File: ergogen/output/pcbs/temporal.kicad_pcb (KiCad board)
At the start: 2 copper layers, 147.9 x 107.9 mm, 57 parts

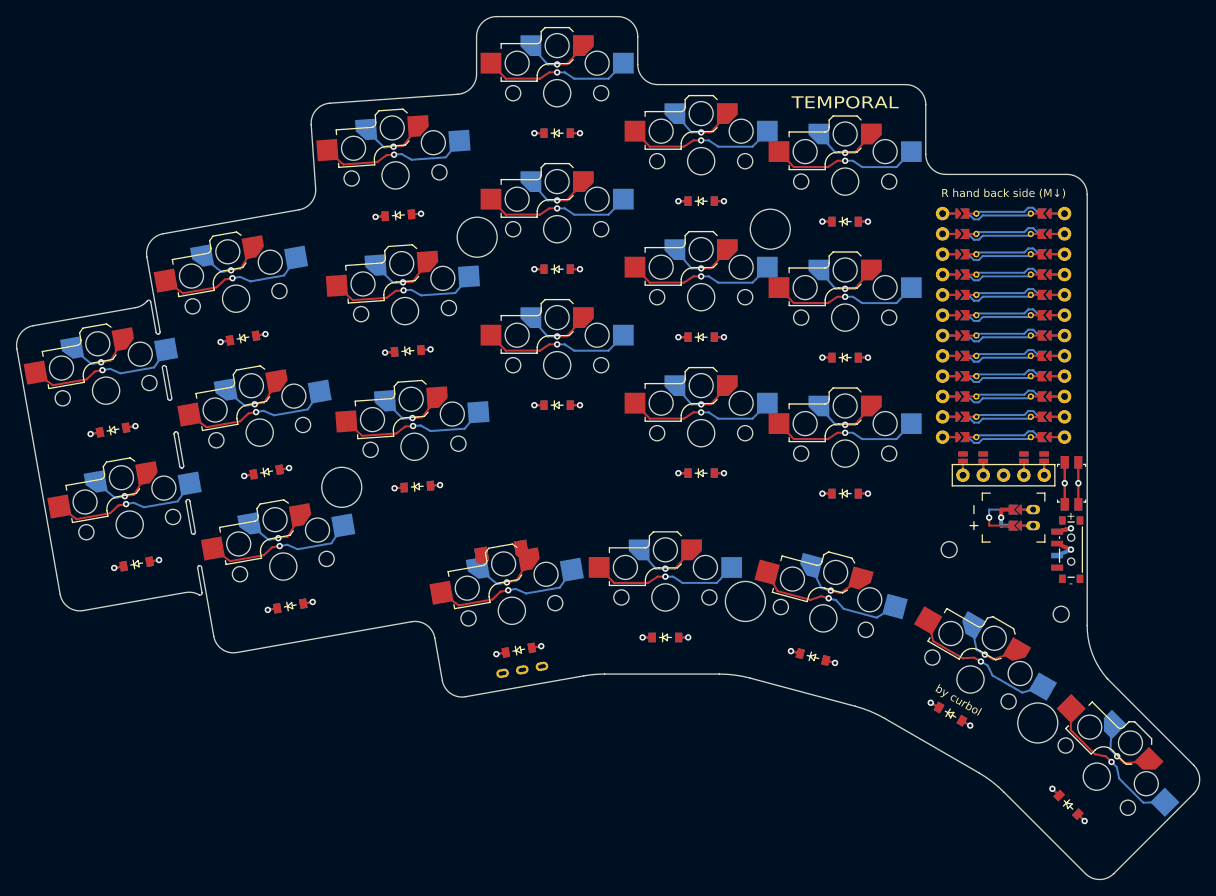
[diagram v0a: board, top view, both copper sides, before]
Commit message: folder cleanup
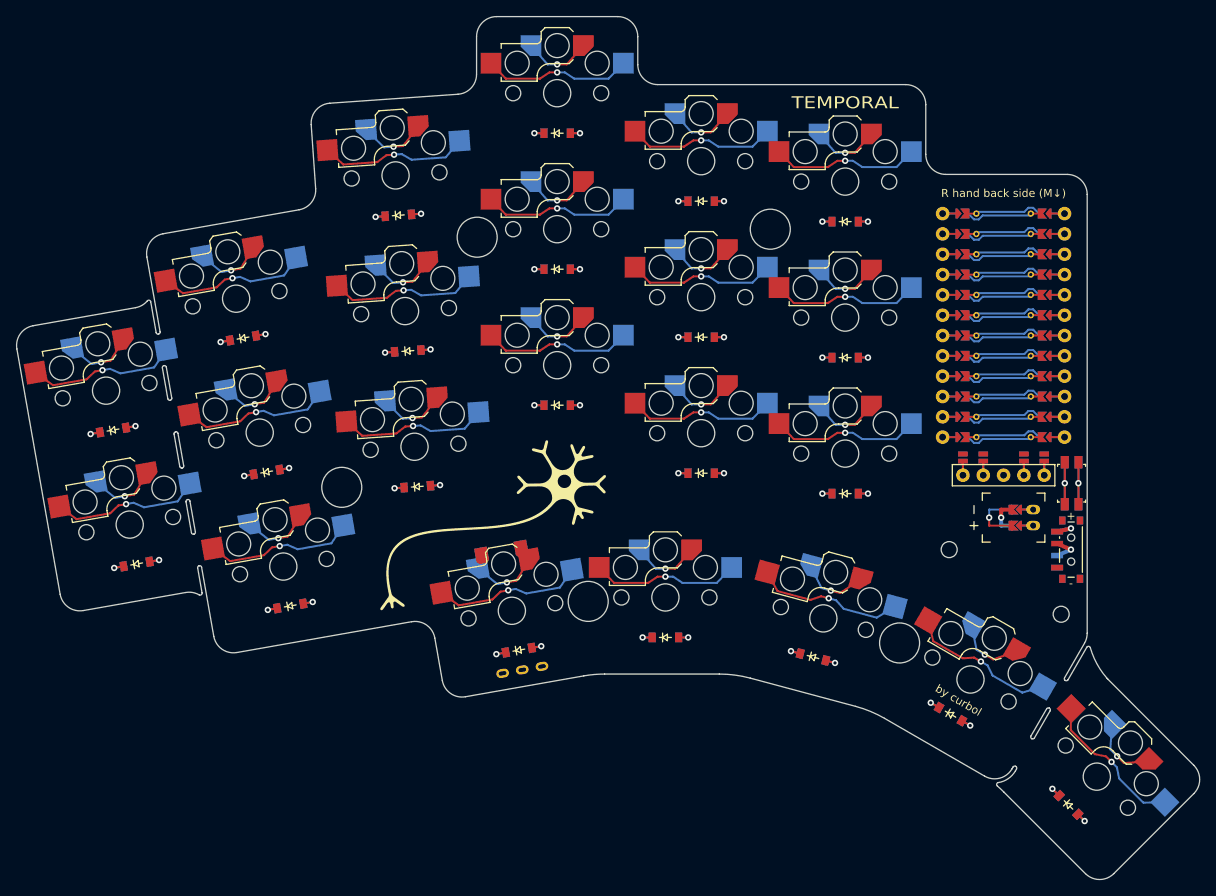
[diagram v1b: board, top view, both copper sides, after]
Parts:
- moved MH3 20.0 mm to (143.3, 98.1), turned to -15 degrees
- moved MH4 19.7 mm to (104.4, 92.9), turned to 10 degrees
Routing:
- net (no net): track 337.7 -> 0.00 mm
- net GND: track 17.9 -> 47.4 mm
- net row_thumb: track 12.0 -> 21.8 mm
- net MOSI: track 0.00 -> 9.84 mm
- net encoder_b: track 0.00 -> 9.84 mm
- net encoder_a: track 0.00 -> 9.84 mm
- net P3: track 0.00 -> 9.84 mm
- net P2: track 0.00 -> 9.84 mm
- net SCK: track 0.00 -> 9.84 mm
- net row_bottom: track 12.0 -> 21.8 mm
- net row_top: track 14.4 -> 24.2 mm
- net row_home: track 14.4 -> 24.2 mm
- net col_ring: track 74.7 -> 84.5 mm
- net col_pinky: track 74.7 -> 84.5 mm
- net col_extra: track 37.3 -> 47.2 mm
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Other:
- outline, holes or cut-outs redrawn
